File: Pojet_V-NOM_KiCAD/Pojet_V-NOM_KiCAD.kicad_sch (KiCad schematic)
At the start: 4 parts

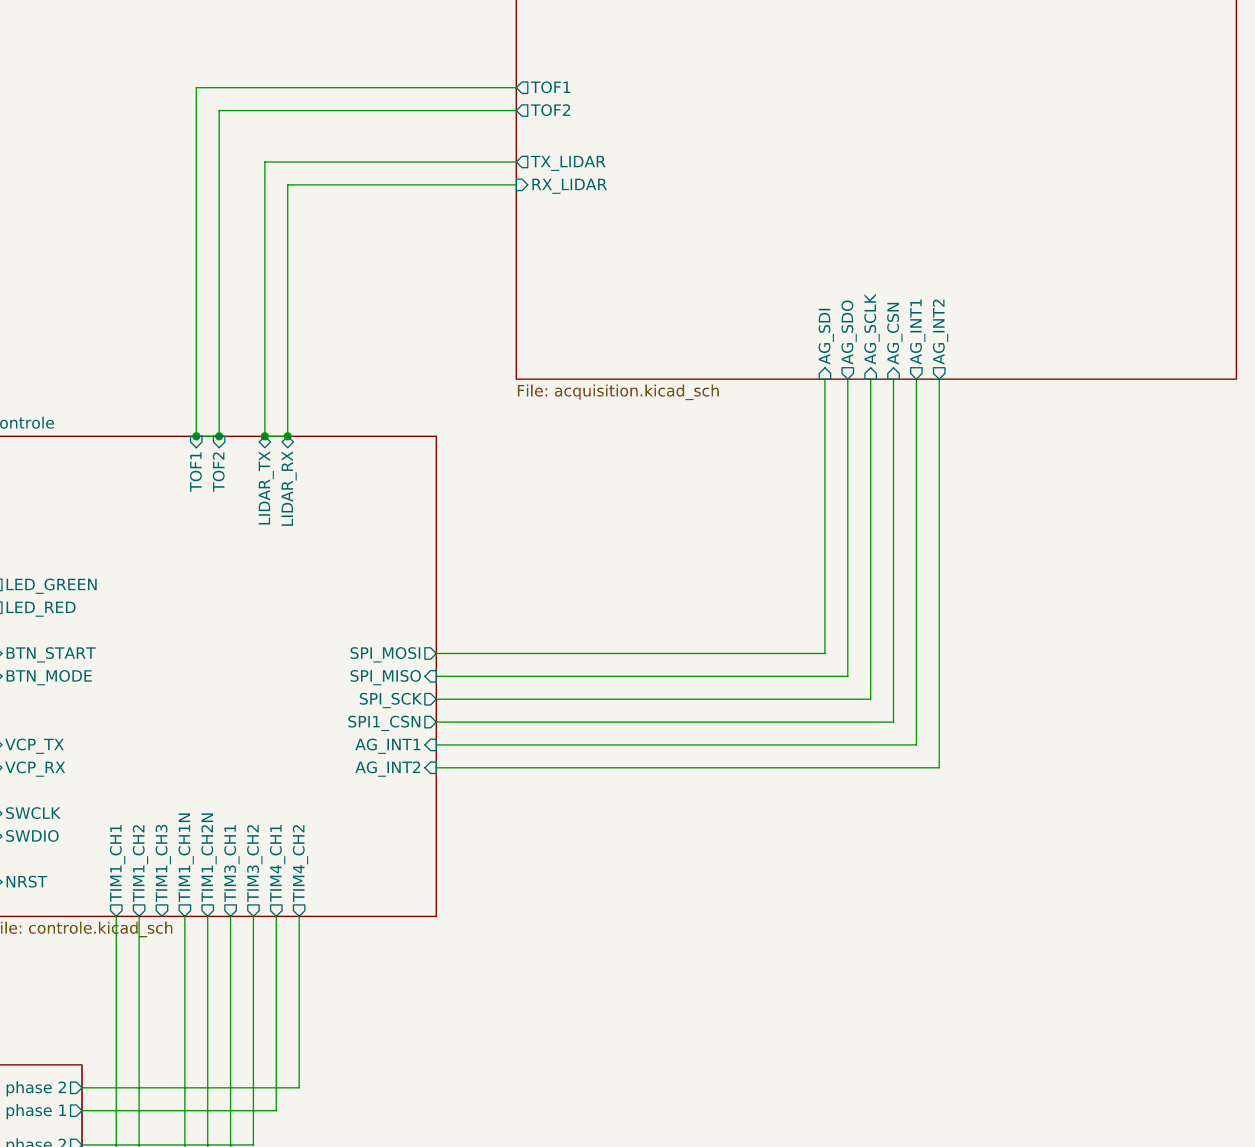
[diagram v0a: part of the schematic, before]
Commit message: Modifications conseillés par l'enseignant
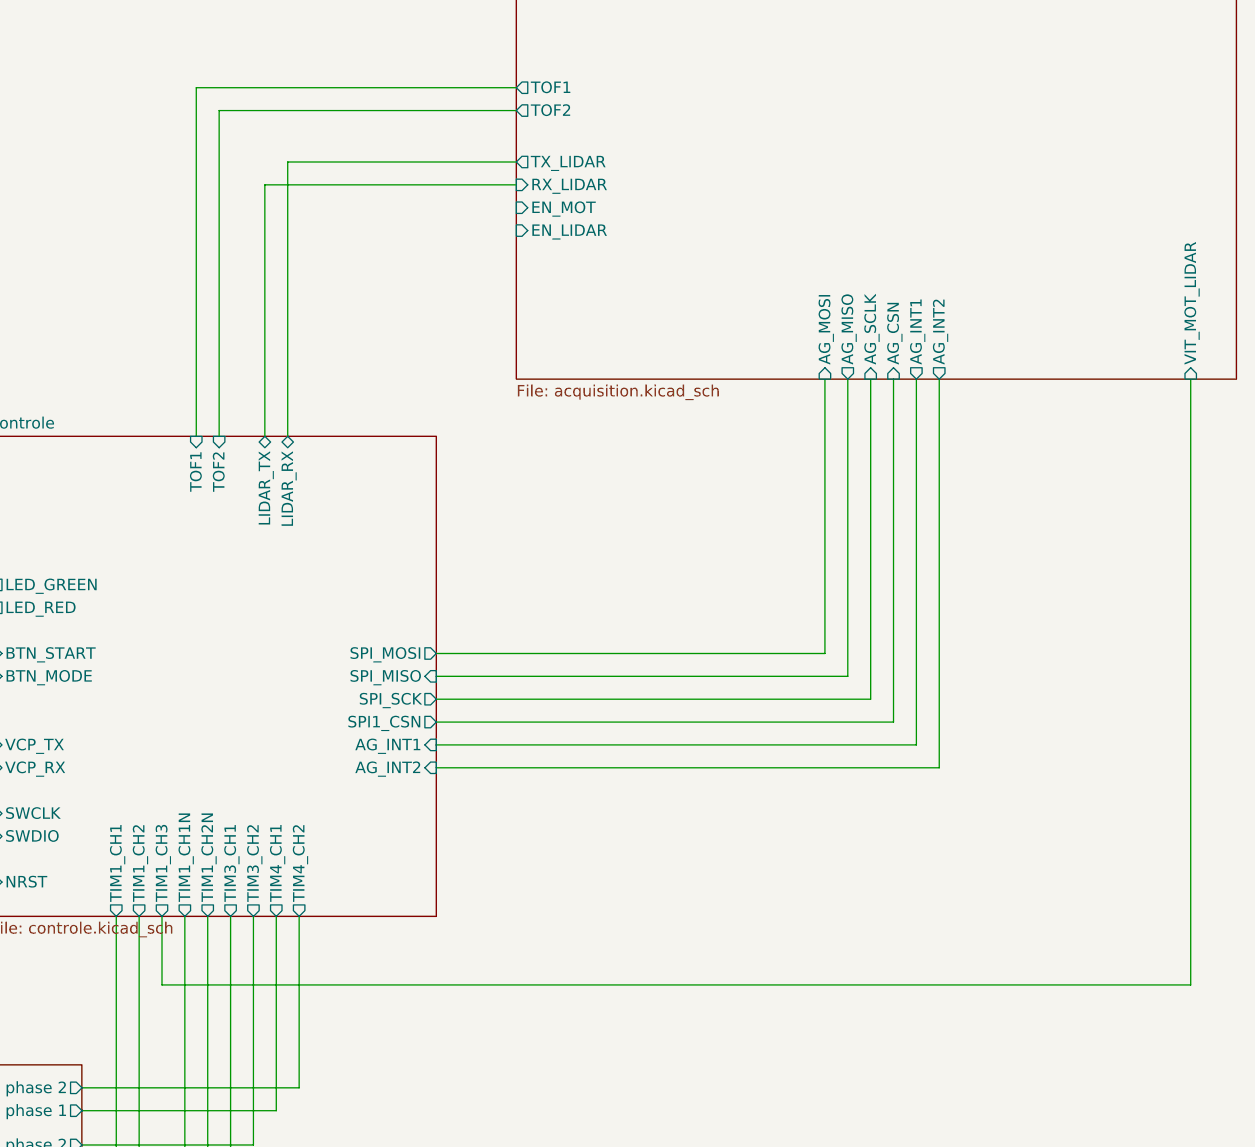
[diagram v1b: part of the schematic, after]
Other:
- sheet acquisition ports: added AG_MISO, AG_MOSI, EN_LIDAR, EN_MOT, VIT_MOT_LIDAR; removed AG_SDI, AG_SDO
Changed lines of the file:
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@@
-	)
-	(junction
-		(at 146.05 71.12)
-		(diameter 0)
-		(color 0 0 0 0)
-	)
-	(junction
-		(at 135.89 71.12)
-		(diameter 0)
-		(color 0 0 0 0)
-	)
-	(junction
-		(at 143.51 71.12)
-		(diameter 0)
-		(color 0 0 0 0)
-	)
-	(junction
-		(at 138.43 71.12)
-		(diameter 0)
-		(color 0 0 0 0)
 	)
 	(junction
@@
 	(wire
 		(pts
-			(xy 143.51 40.64) (xy 171.45 40.64)
-		)
-		(stroke
-			(width 0)
-			(type default)
-		)
-	)
-	(wire
-		(pts
 			(xy 134.62 167.64) (xy 123.19 167.64)
 		)
@@
 	(wire
 		(pts
-			(xy 146.05 43.18) (xy 171.45 43.18)
+			(xy 132.08 124.46) (xy 132.08 132.08)
 		)
 		(stroke
@@
 	(wire
 		(pts
+			(xy 246.38 132.08) (xy 246.38 64.77)
+		)
+		(stroke
+			(width 0)
+			(type default)
+		)
+	)
+	(wire
+		(pts
 			(xy 86.36 115.57) (xy 113.03 115.57)
 		)
@@
 	(wire
 		(pts
+			(xy 171.45 40.64) (xy 146.05 40.64)
+		)
+		(stroke
+			(width 0)
+			(type default)
+		)
+	)
+	(wire
+		(pts
 			(xy 208.28 64.77) (xy 208.28 97.79)
 		)
@@
 	(wire
 		(pts
-			(xy 146.05 71.12) (xy 146.05 43.18)
-		)
-		(stroke
-			(width 0)
-			(type default)
-		)
-	)
-	(wire
-		(pts
 			(xy 129.54 157.48) (xy 123.19 157.48)
 		)
@@
 	(wire
 		(pts
+			(xy 146.05 40.64) (xy 146.05 71.12)
+		)
+		(stroke
+			(width 0)
+			(type default)
+		)
+	)
+	(wire
+		(pts
 			(xy 86.36 95.25) (xy 113.03 95.25)
 		)
@@
 	(wire
 		(pts
-			(xy 146.05 71.12) (xy 143.51 71.12)
-		)
-		(stroke
-			(width 0)
-			(type default)
-		)
-	)
-	(wire
-		(pts
 			(xy 86.36 105.41) (xy 113.03 105.41)
 		)
@@
 	(wire
 		(pts
-			(xy 138.43 71.12) (xy 135.89 71.12)
-		)
-		(stroke
-			(width 0)
-			(type default)
-		)
-	)
-	(wire
-		(pts
 			(xy 215.9 64.77) (xy 215.9 105.41)
 		)
@@
 	(wire
 		(pts
+			(xy 132.08 132.08) (xy 246.38 132.08)
+		)
+		(stroke
+			(width 0)
+			(type default)
+		)
+	)
+	(wire
+		(pts
 			(xy 123.19 149.86) (xy 142.24 149.86)
 		)
@@
 	(wire
 		(pts
-			(xy 143.51 71.12) (xy 143.51 40.64)
+			(xy 143.51 43.18) (xy 143.51 71.12)
 		)
 		(stroke
@@
 		(pts
 			(xy 213.36 64.77) (xy 213.36 102.87)
+		)
+		(stroke
+			(width 0)
+			(type default)
+		)
+	)
+	(wire
+		(pts
+			(xy 171.45 43.18) (xy 143.51 43.18)
 		)
 		(stroke
@@
 			)
 		)
-		(pin "AG_SDI" input
+		(pin "EN_MOT" input
+			(at 171.45 45.72 180)
+			(effects
+				(font
+					(size 1.27 1.27)
+				)
+				(justify left)
+			)
+		)
+		(pin "EN_LIDAR" input
+			(at 171.45 48.26 180)
+			(effects
+				(font
+					(size 1.27 1.27)
+				)
+				(justify left)
+			)
+		)
+		(pin "VIT_MOT_LIDAR" input
+			(at 246.38 64.77 270)
+			(effects
+				(font
+					(size 1.27 1.27)
+				)
+				(justify left)
+			)
+		)
+		(pin "AG_MOSI" input
 			(at 205.74 64.77 270)
 			(effects
@@
 			)
 		)
-		(pin "AG_SDO" output
+		(pin "AG_MISO" output
 			(at 208.28 64.77 270)
 			(effects
